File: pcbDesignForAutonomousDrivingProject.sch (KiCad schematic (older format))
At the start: 3 parts

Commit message: Commit Made on - April 17th 2021 @ 01:57:31 PM
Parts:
- removed J?: ExternalDAC, symbol myComponents:ExternalDAC
- removed J?: Conn_01x04, symbol Connector_Generic:Conn_01x04
- added U? (x5): ultrasonic, symbol myComponents:ultrasonic
- added U?: can, symbol myComponents:can
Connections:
- net labels added: 3.3v, 5v, GND, SCL, SDA, canRX, canTx
- no-connect marks 0 -> 35
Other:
- moved on the sheet: U?
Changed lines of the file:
@@
 L myComponents:SJ2Board U?
 U 1 1 607A89AA
-P 2200 2300
-F 0 "U?" H 2200 3465 50  0000 C CNN
-F 1 "SJ2Board" H 2200 3374 50  0000 C CNN
-F 2 "" H 2200 1300 50  0001 C CNN
-F 3 "" H 2200 1300 50  0001 C CNN
-	1    2200 2300
+P 2600 2100
+F 0 "U?" H 2600 3265 50  0000 C CNN
+F 1 "SJ2Board" H 2600 3174 50  0000 C CNN
+F 2 "" H 2600 1100 50  0001 C CNN
+F 3 "" H 2600 1100 50  0001 C CNN
+	1    2600 2100
 	1    0    0    -1
 $EndComp
 $Comp
-L myComponents:ExternalDAC J?
-U 1 1 607E8440
-P 2200 4100
-F 0 "J?" H 2588 4164 50  0000 L CNN
-F 1 "ExternalDAC" H 2588 4073 50  0000 L CNN
-F 2 "" V 2200 4200 50  0001 C CNN
-F 3 "~" V 2200 4200 50  0001 C CNN
-	1    2200 4100
-	1    0    0    -1
+L myComponents:ultrasonic U?
+U 1 1 607B7CAD
+P 3600 1200
+F 0 "U?" V 3628 1428 50  0000 L CNN
+F 1 "ultrasonic" V 3695 1428 20  0000 L CNN
+F 2 "" H 3100 900 50  0001 C CNN
+F 3 "" H 3100 900 50  0001 C CNN
+	1    3600 1200
+	0    1    1    0
 $EndComp
 $Comp
-L Connector_Generic:Conn_01x04 J?
-U 1 1 607E9889
-P 1300 3100
-F 0 "J?" H 1380 3092 50  0000 L CNN
-F 1 "Conn_01x04" H 1380 3001 50  0000 L CNN
-F 2 "" H 1300 3100 50  0001 C CNN
-F 3 "~" H 1300 3100 50  0001 C CNN
-	1    1300 3100
-	1    0    0    -1
+L myComponents:ultrasonic U?
+U 1 1 607B88FD
+P 4300 1200
+F 0 "U?" V 4328 1428 50  0000 L CNN
+F 1 "ultrasonic" V 4395 1428 20  0000 L CNN
+F 2 "" H 3800 900 50  0001 C CNN
+F 3 "" H 3800 900 50  0001 C CNN
+	1    4300 1200
+	0    1    1    0
 $EndComp
+$Comp
+L myComponents:ultrasonic U?
+U 1 1 607B8C42
+P 5000 1200
+F 0 "U?" V 5028 1428 50  0000 L CNN
+F 1 "ultrasonic" V 5095 1428 20  0000 L CNN
+F 2 "" H 4500 900 50  0001 C CNN
+F 3 "" H 4500 900 50  0001 C CNN
+	1    5000 1200
+	0    1    1    0
+$EndComp
+$Comp
+L myComponents:ultrasonic U?
+U 1 1 607B8E5B
+P 5700 1200
+F 0 "U?" V 5728 1428 50  0000 L CNN
+F 1 "ultrasonic" V 5795 1428 20  0000 L CNN
+F 2 "" H 5200 900 50  0001 C CNN
+F 3 "" H 5200 900 50  0001 C CNN
+	1    5700 1200
+	0    1    1    0
+$EndComp
+$Comp
+L myComponents:ultrasonic U?
+U 1 1 607B9182
+P 6300 1200
+F 0 "U?" V 6328 1428 50  0000 L CNN
+F 1 "ultrasonic" V 6395 1428 20  0000 L CNN
+F 2 "" H 5800 900 50  0001 C CNN
+F 3 "" H 5800 900 50  0001 C CNN
+	1    6300 1200
+	0    1    1    0
+$EndComp
+Text GLabel 3500 1300 0    39   Input ~ 0
+SCL
+Text GLabel 4200 1300 0    39   Input ~ 0
+SCL
+Text GLabel 4900 1300 0    39   Input ~ 0
+SCL
+Text GLabel 5600 1300 0    39   Input ~ 0
+SCL
+Text GLabel 3500 1400 0    39   Input ~ 0
+SDA
+Text GLabel 4200 1400 0    39   Input ~ 0
+SDA
+Text GLabel 4900 1400 0    39   Input ~ 0
+SDA
+Text GLabel 5600 1400 0    39   Input ~ 0
+SDA
+Text GLabel 3100 3000 2    39   Input ~ 0
+SCL
+Text GLabel 6200 1300 0    39   Input ~ 0
+SCL
+Text GLabel 6200 1400 0    39   Input ~ 0
+SDA
+Text GLabel 2100 3000 0    39   Input ~ 0
+SDA
+Text GLabel 3500 1100 0    39   Input ~ 0
+3.3v
+Text GLabel 4200 1100 0    39   Input ~ 0
+3.3v
+Text GLabel 4900 1100 0    39   Input ~ 0
+3.3v
+Text GLabel 5600 1100 0    39   Input ~ 0
+3.3v
+Text GLabel 6200 1100 0    39   Input ~ 0
+3.3v
+Text GLabel 3500 1200 0    39   Input ~ 0
+GND
+Text GLabel 4200 1200 0    39   Input ~ 0
+GND
+Text GLabel 4900 1200 0    39   Input ~ 0
+GND
+Text GLabel 5600 1200 0    39   Input ~ 0
+GND
+Text GLabel 6200 1200 0    39   Input ~ 0
+GND
+Text GLabel 3100 1200 2    39   Input ~ 0
+5v
+NoConn ~ 3100 1300
+NoConn ~ 3100 1400
+NoConn ~ 3100 1500
+NoConn ~ 3100 1600
+NoConn ~ 3100 1700
+NoConn ~ 3100 1800
+NoConn ~ 3100 1900
+NoConn ~ 3100 2000
+NoConn ~ 3100 2500
+NoConn ~ 3100 2400
+NoConn ~ 3100 2600
+NoConn ~ 3100 2800
+NoConn ~ 3100 2700
+NoConn ~ 3100 2900
+NoConn ~ 3100 2100
+NoConn ~ 3100 2200
+NoConn ~ 3100 2300
+NoConn ~ 2100 2900
+NoConn ~ 2100 2800
+NoConn ~ 2100 2700
+NoConn ~ 2100 2600
+NoConn ~ 2100 2500
+NoConn ~ 2100 2400
+NoConn ~ 2100 2300
+NoConn ~ 2100 2200
+NoConn ~ 2100 2100
+NoConn ~ 2100 2000
+NoConn ~ 2100 1900
+NoConn ~ 2100 1800
+NoConn ~ 2100 1700
+NoConn ~ 2100 1600
+NoConn ~ 2100 1200
+NoConn ~ 2100 1300
+NoConn ~ 2100 1400
+NoConn ~ 2100 1500
+Text GLabel 3100 3100 2    39   Input ~ 0
+GND
+Text GLabel 2100 3100 0    39   Input ~ 0
+GND
+Wire Notes Line
+	500  600  6900 600
+Wire Notes Line
+	6900 600  6900 1900
+Wire Notes Line
+	6900 1900 3700 1900
+Wire Notes Line
+	3700 1900 3700 3500
+Wire Notes Line
+	3700 3500 500  3500
+Wire Notes Line
+	500  3500 500  600
+Text GLabel 1700 1400 2    39   Input ~ 0
+GND
+Text GLabel 1700 1300 2    39   Input ~ 0
+3.3v
+Text GLabel 1700 1500 2    39   Input ~ 0
+canRX
+$Comp
+L myComponents:can U?
+U 1 1 607BC269
+P 1100 1400
+F 0 "U?" V 1465 1300 50  0000 C CNN
+F 1 "can" V 1374 1300 50  0000 C CNN
+F 2 "" H 600 2100 50  0001 C CNN
+F 3 "" H 600 2100 50  0001 C CNN
+	1    1100 1400
+	0    -1   -1   0
+$EndComp
+Text GLabel 1700 1600 2    39   Input ~ 0
+canTx
 $EndSCHEMATC

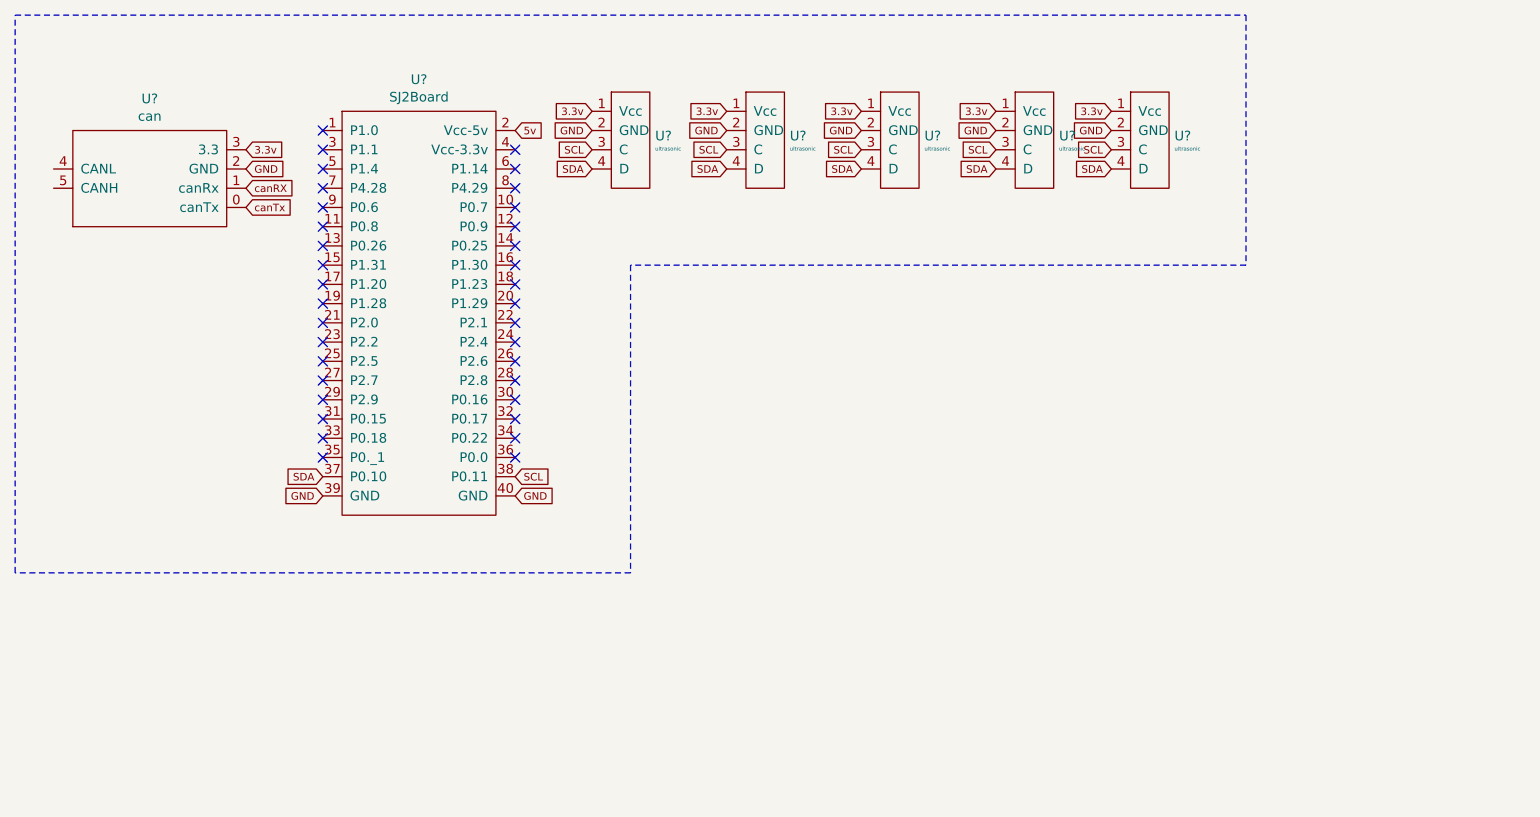
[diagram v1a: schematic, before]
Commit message: Commit Made on - April 18th 2021 @ 04:05:23 PM
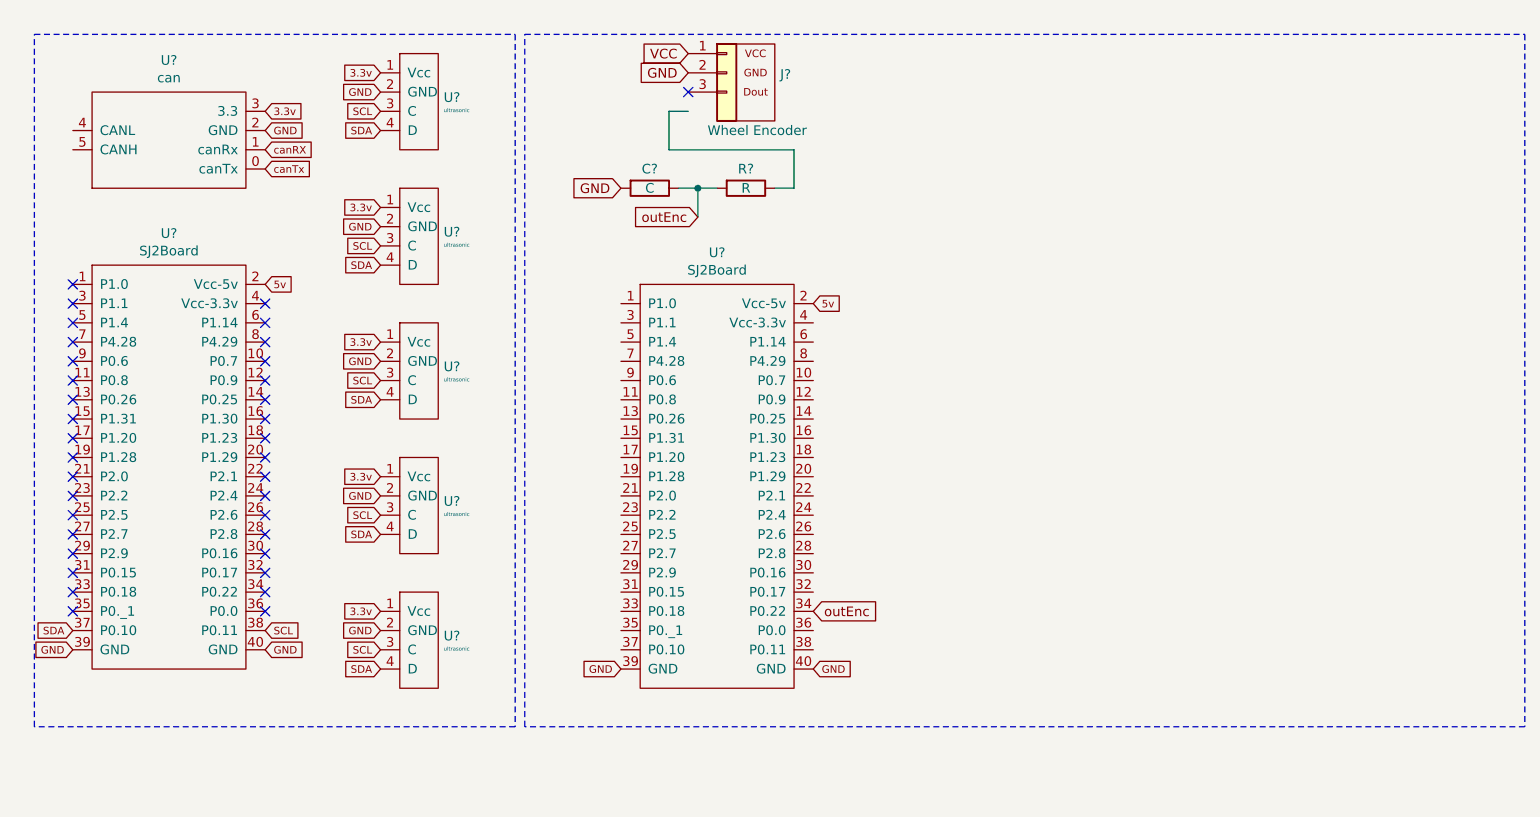
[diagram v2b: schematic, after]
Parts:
- added C?: C, symbol Device:R
- added J?: Wheel Encoder, symbol myComponents:Encoder
- added R?: R, symbol Device:R
- added U?: SJ2Board, symbol myComponents:SJ2Board
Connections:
- net labels added: VCC, outEnc
- wire segments 0 -> 8
- no-connect marks 35 -> 36
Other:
- moved on the sheet: U?
